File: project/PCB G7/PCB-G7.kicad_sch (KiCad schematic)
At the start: 19 parts, among them J1 Micro_SD_Card, J10 jumper 2, J11 jumper 1, J12 jumper 2, J3 Oled, J4 servomoteur, J5 stepper 1, J6 stepper 2, J7 Barrel_Jack_Switch, J8 jumper 1, U2 ESP32-S3-UNO

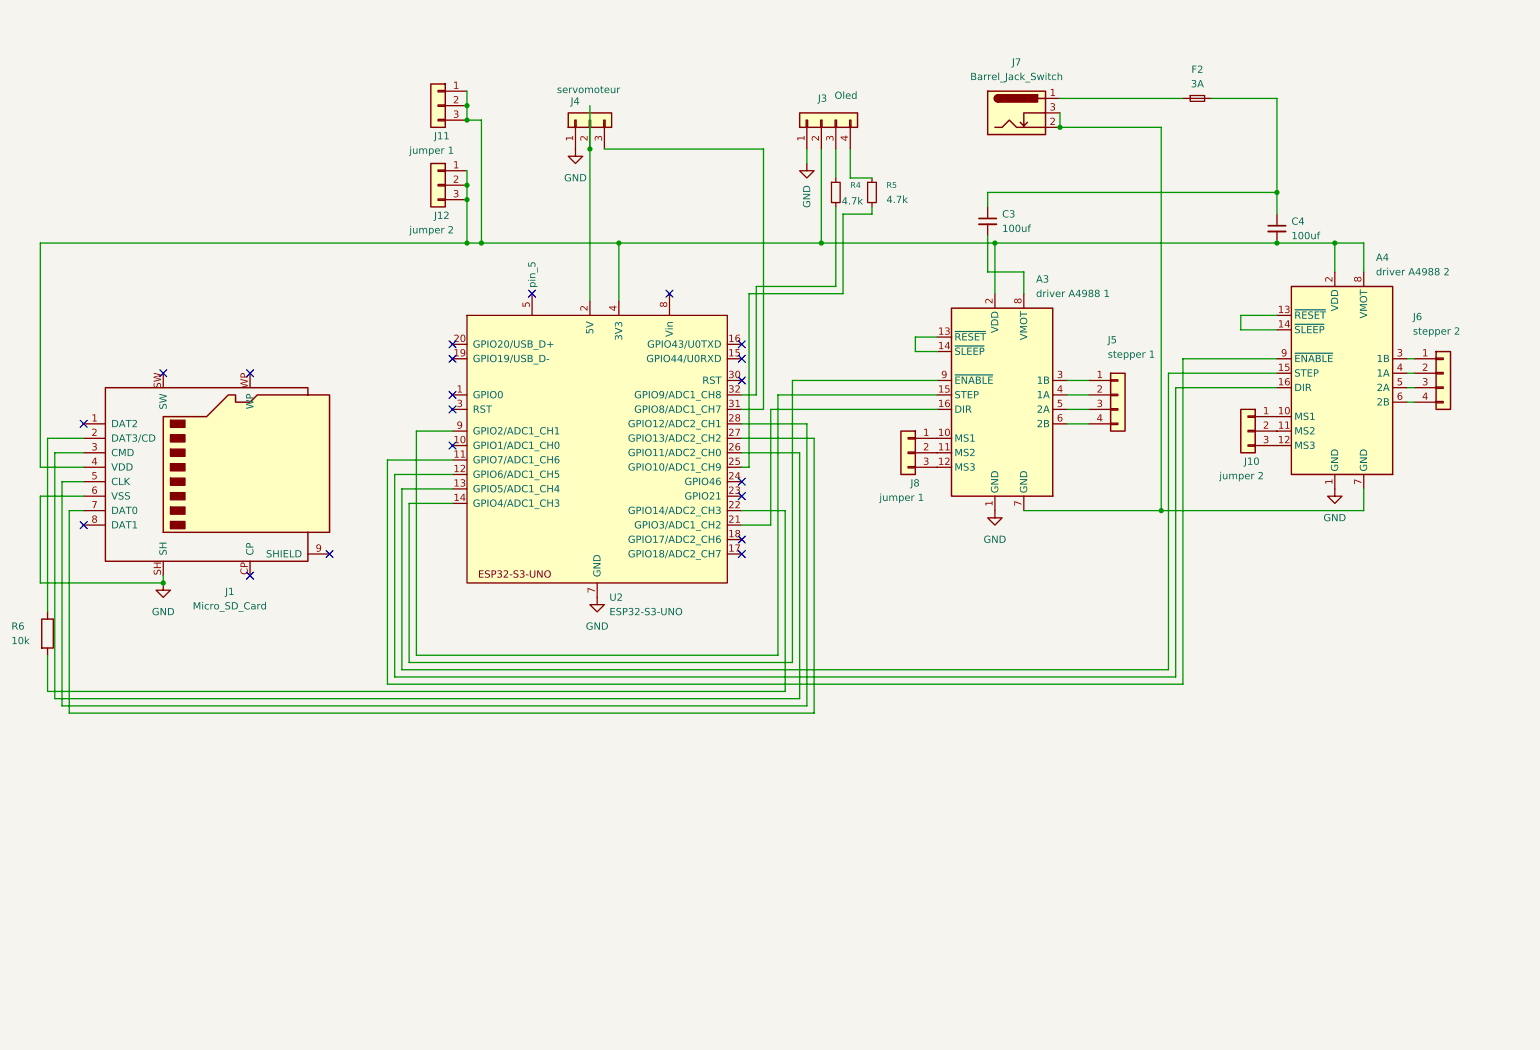
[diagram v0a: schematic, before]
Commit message: update schematics et pcb
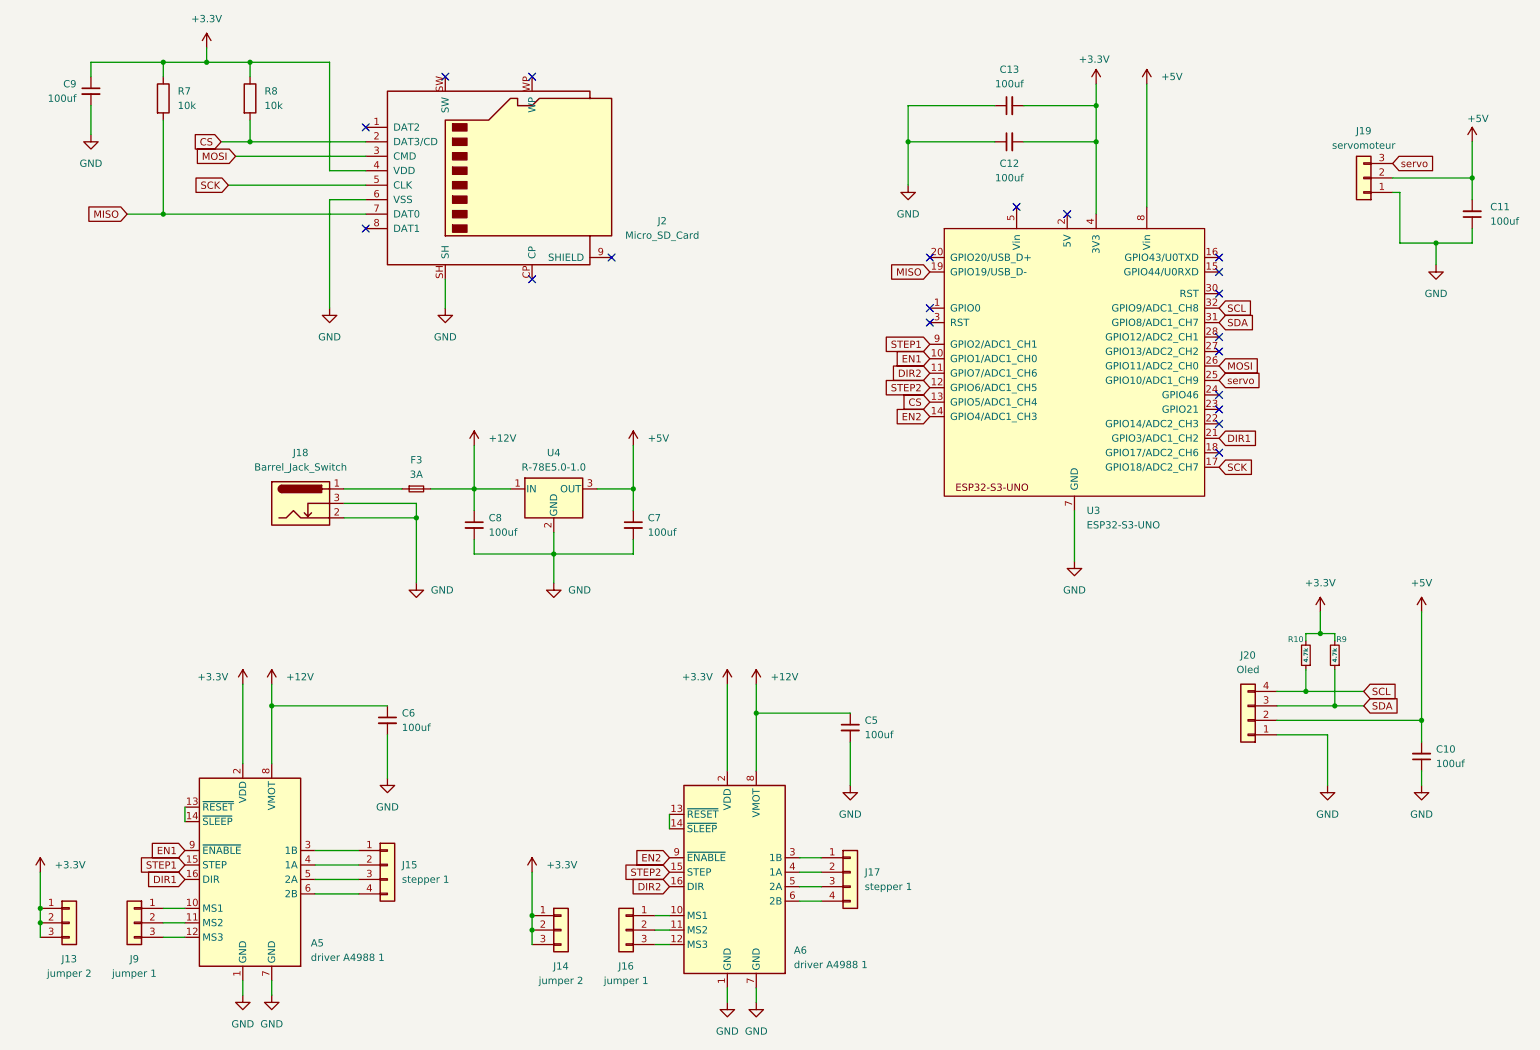
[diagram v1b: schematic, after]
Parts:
- removed A3: driver A4988 1, Module:Pololu_Breakout-16_15.2x20.3mm, symbol Driver_Motor:Pololu_Breakout_A4988
- removed A4: driver A4988 2, Module:Pololu_Breakout-16_15.2x20.3mm, symbol Driver_Motor:Pololu_Breakout_A4988
- removed C3, C4: 100uf, symbol makerspace-unilasalle:C
- removed F2: 3A, Fuse:Fuseholder_Blade_Mini_Keystone_3568, symbol makerspace-unilasalle:Fuse
- removed J1: Micro_SD_Card, Connector_Card:SD_Hirose_DM1AA_SF_PEJ82, symbol Connector:Micro_SD_Card
- removed J10, J12: jumper 2, symbol makerspace-unilasalle:Conn_01x03
- removed J11, J8: jumper 1, symbol makerspace-unilasalle:Conn_01x03
- removed J3: Oled, Display:OLED-128O064D, symbol makerspace-unilasalle:Conn_01x04
- removed J4: servomoteur, symbol makerspace-unilasalle:Conn_01x03
- removed J5: stepper 1, symbol makerspace-unilasalle:Conn_01x04
- removed J6: stepper 2, symbol makerspace-unilasalle:Conn_01x04
- removed J7: Barrel_Jack_Switch, symbol makerspace-unilasalle:Barrel_Jack_Switch
- removed R4, R5: 4.7k, symbol makerspace-unilasalle:R
- removed R6: 10k, Resistor_THT:R_Axial_DIN0207_L6.3mm_D2.5mm_P10.16mm_Horizontal, symbol Device:R
- removed U2: ESP32-S3-UNO, makerspace-unilasalle:ESP_S3_UNO, symbol makerspace-unilasalle:ESP32-S3-UNO
- added A5, A6: driver A4988 1, Module:Pololu_Breakout-16_15.2x20.3mm, symbol Driver_Motor:Pololu_Breakout_A4988
- added C10, C11, C12, C13, C5, C6, C9: 100uf, symbol makerspace-unilasalle:C
- added C7, C8: 100uf, Capacitor_SMD:C_1206_3216Metric_Pad1.33x1.80mm_HandSolder, symbol makerspace-unilasalle:C
- added F3: 3A, Fuse:Fuseholder_Blade_Mini_Keystone_3568, symbol makerspace-unilasalle:Fuse
- added J13, J14: jumper 2, symbol makerspace-unilasalle:Conn_01x03
- added J15, J17: stepper 1, symbol makerspace-unilasalle:Conn_01x04
- added J16, J9: jumper 1, symbol makerspace-unilasalle:Conn_01x03
- added J18: Barrel_Jack_Switch, symbol makerspace-unilasalle:Barrel_Jack_Switch
- added J19: servomoteur, symbol makerspace-unilasalle:Conn_01x03
- added J2: Micro_SD_Card, Connector_Card:SD_Hirose_DM1AA_SF_PEJ82, symbol Connector:Micro_SD_Card
- added J20: Oled, Display:OLED-128O064D, symbol makerspace-unilasalle:Conn_01x04
- added R10, R9: 4.7k, symbol makerspace-unilasalle:R
- added R7, R8: 10k, Resistor_THT:R_Axial_DIN0207_L6.3mm_D2.5mm_P10.16mm_Horizontal, symbol Device:R
- added U3: ESP32-S3-UNO, makerspace-unilasalle:ESP_S3_UNO, symbol makerspace-unilasalle:ESP32-S3-UNO
- added U4: R-78E5.0-1.0, Converter_DCDC:Converter_DCDC_RECOM_R-78E-0.5_THT, symbol makerspace-unilasalle:R-78E5.0-1.0
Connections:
- net GND: now also A5.1 (GND), A5.7 (GND), A6.1 (GND), A6.7 (GND), C10.1, C11.1, C12.1, C13.1, C5.2, C6.2, C7.2, C8.2, C9.2, J18.2, J18.3, J19.1 (Pin_1), J2.6 (VSS), J2.SH, J20.1 (Pin_1), U3.29 (GND), U3.6 (GND), U3.7 (GND), U4.2 (GND)
- new net: A5.10 (MS1), J9.1 (Pin_1)
- new net: A5.11 (MS2), J9.2 (Pin_2)
- new net: A5.12 (MS3), J9.3 (Pin_3)
- new net: A6.10 (MS1), J16.1 (Pin_1)
- new net: A6.11 (MS2), J16.2 (Pin_2)
- new net: A6.12 (MS3), J16.3 (Pin_3)
- new net: A6.13 (~{RESET}), A6.14 (~{SLEEP})
- new net: A6.3 (1B), J17.1 (Pin_1)
- new net: A6.4 (1A), J17.2 (Pin_2)
- new net: A6.5 (2A), J17.3 (Pin_3)
- new net: A6.6 (2B), J17.4 (Pin_4)
- new net: F3.1, J18.1
- new net: A5.3 (1B), J15.1 (Pin_1)
- new net: A5.4 (1A), J15.2 (Pin_2)
- new net: A5.5 (2A), J15.3 (Pin_3)
- new net: A5.6 (2B), J15.4 (Pin_4)
- new net: A5.13 (~{RESET}), A5.14 (~{SLEEP})
- new net +12V: A5.8 (VMOT), A6.8 (VMOT), C5.1, C6.1, C8.1, F3.2, U4.1 (IN)
- new net +3.3V: A5.2 (VDD), A6.2 (VDD), C12.2, C13.2, C9.1, J13.1 (Pin_1), J13.2 (Pin_2), J13.3 (Pin_3), J14.1 (Pin_1), J14.2 (Pin_2), J14.3 (Pin_3), J2.4 (VDD), R10.2, R7.1, R8.1, R9.2, U3.4 (3V3)
- new net +5V: C10.2, C11.2, C7.1, J19.2 (Pin_2), J20.2 (Pin_2), U3.8 (Vin), U4.3 (OUT)
- new net CS: J2.2 (DAT3/CD), R8.2, U3.13 (GPIO5/ADC1_CH4)
- new net DIR1: A5.16 (DIR), U3.21 (GPIO3/ADC1_CH2)
- new net DIR2: A6.16 (DIR), U3.11 (GPIO7/ADC1_CH6)
- new net EN1: A5.9 (~{ENABLE}), U3.10 (GPIO1/ADC1_CH0)
- new net EN2: A6.9 (~{ENABLE}), U3.14 (GPIO4/ADC1_CH3)
- new net MISO: J2.7 (DAT0), R7.2, U3.19 (GPIO19/USB_D-)
- new net MOSI: J2.3 (CMD), U3.26 (GPIO11/ADC2_CH0)
- new net SCK: J2.5 (CLK), U3.17 (GPIO18/ADC2_CH7)
- new net SCL: J20.4 (Pin_4), R10.1, U3.32 (GPIO9/ADC1_CH8)
- new net SDA: J20.3 (Pin_3), R9.1, U3.31 (GPIO8/ADC1_CH7)
- new net STEP1: A5.15 (STEP), U3.9 (GPIO2/ADC1_CH1)
- new net STEP2: A6.15 (STEP), U3.12 (GPIO6/ADC1_CH5)
- new net servo: J19.3 (Pin_3), U3.25 (GPIO10/ADC1_CH9)
